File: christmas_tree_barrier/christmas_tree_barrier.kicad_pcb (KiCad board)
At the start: 2 copper layers, 15 parts, among them CON1 AVR-ISP-6, IC1 MIC5225-3.3, J1 USB_OTG, J2 JSTPH, J3 JSTPH, Q1 Q_PNP_BEC, U1 ATTINY45-20SU, Y1 8Mhz

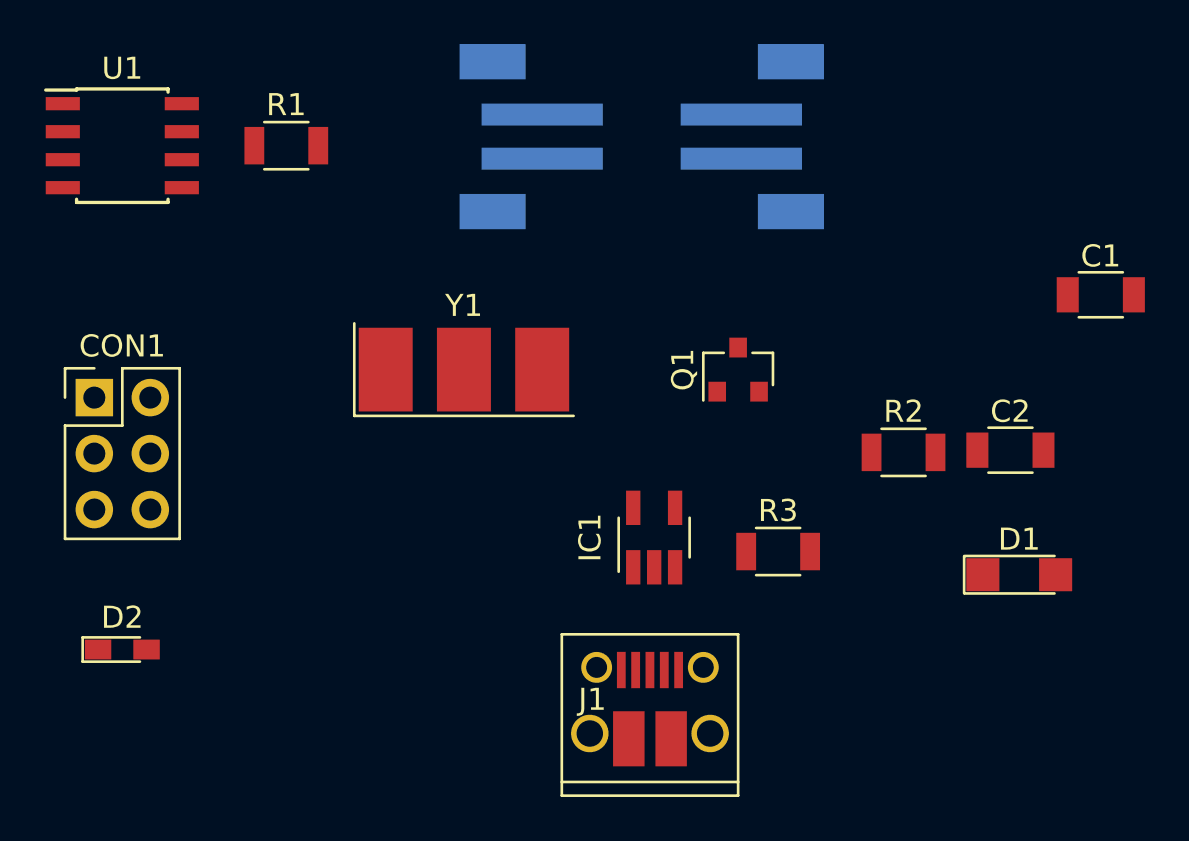
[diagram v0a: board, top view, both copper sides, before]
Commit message: Place parts nicely
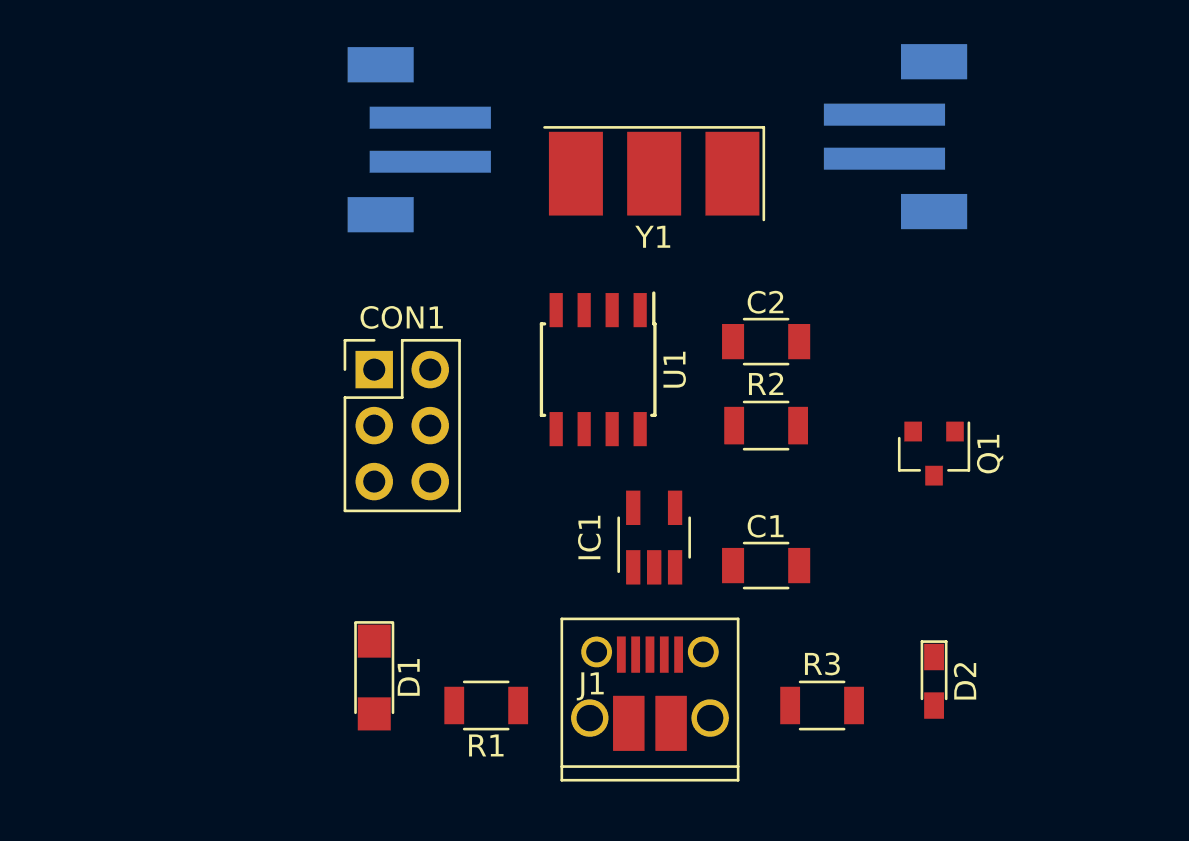
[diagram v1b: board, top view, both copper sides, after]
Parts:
- moved D2 36.9 mm to (172.7, 129.7), turned to 270 degrees
- moved D1 29.6 mm to (147.3, 129.5), turned to 270 degrees
- moved R1 27.0 mm to (152.4, 130.8), turned to 180 degrees
- moved U1 23.9 mm to (157.5, 115.6), turned to 270 degrees
- moved C1 19.5 mm to (165.1, 124.5)
- moved CON1 12.8 mm to (147.3, 115.6)
- moved Y1 12.4 mm to (160.0, 106.7), turned to 180 degrees
- moved C2 12.1 mm to (165.1, 114.3)
- moved Q1 9.67 mm to (172.7, 119.4), turned to 270 degrees
- moved R3 7.26 mm to (167.6, 130.8)
- moved J3 6.50 mm to (171.6, 105.0)
- moved R2 6.35 mm to (165.1, 118.1)
- moved J2 5.08 mm to (148.7, 105.1)
- moved J1 0.70 mm to (159.8, 130.0)
